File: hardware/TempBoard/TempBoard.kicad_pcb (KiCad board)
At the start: 2 copper layers, 27.1 x 27.1 mm, 17 parts, among them J1 Conn_01x04, J2 Conn_01x03, U1 BME280

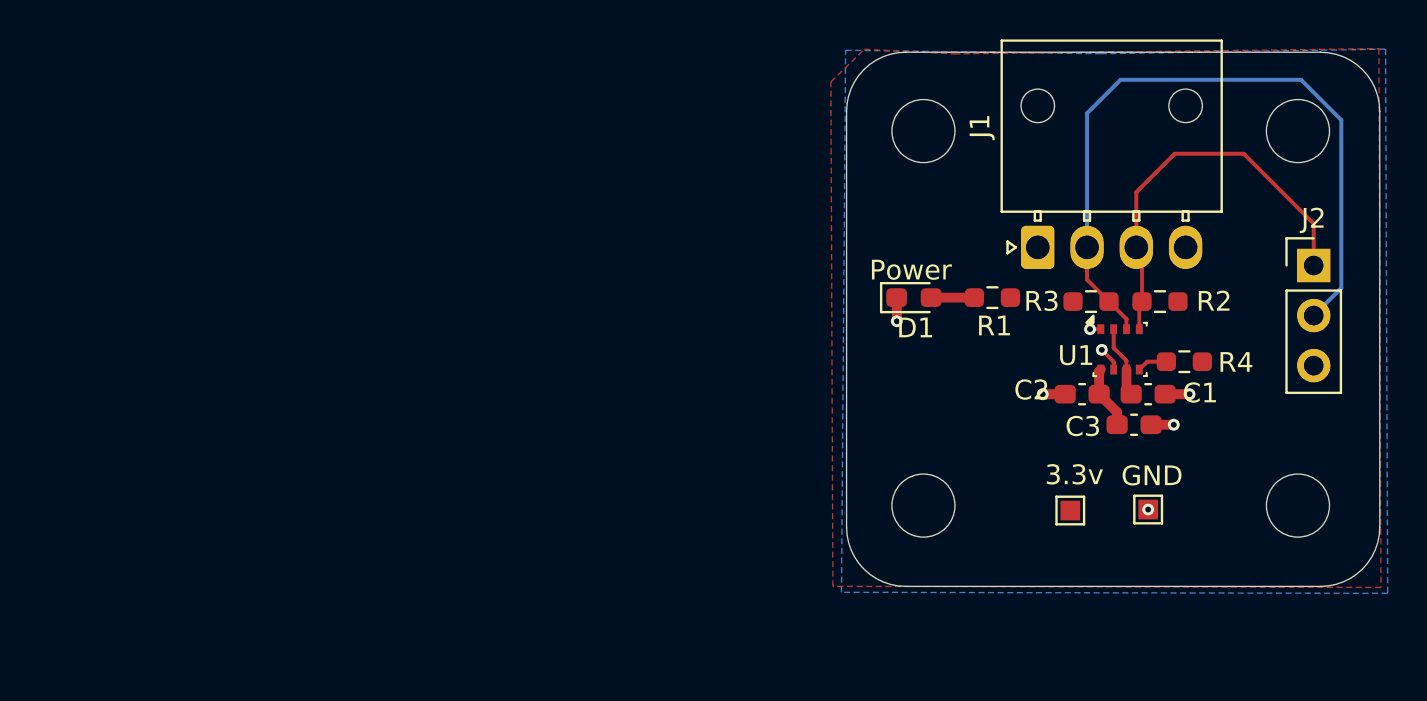
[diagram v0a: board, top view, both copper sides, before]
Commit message: pitot board ordered, routing+size finished for temperature board so pull??
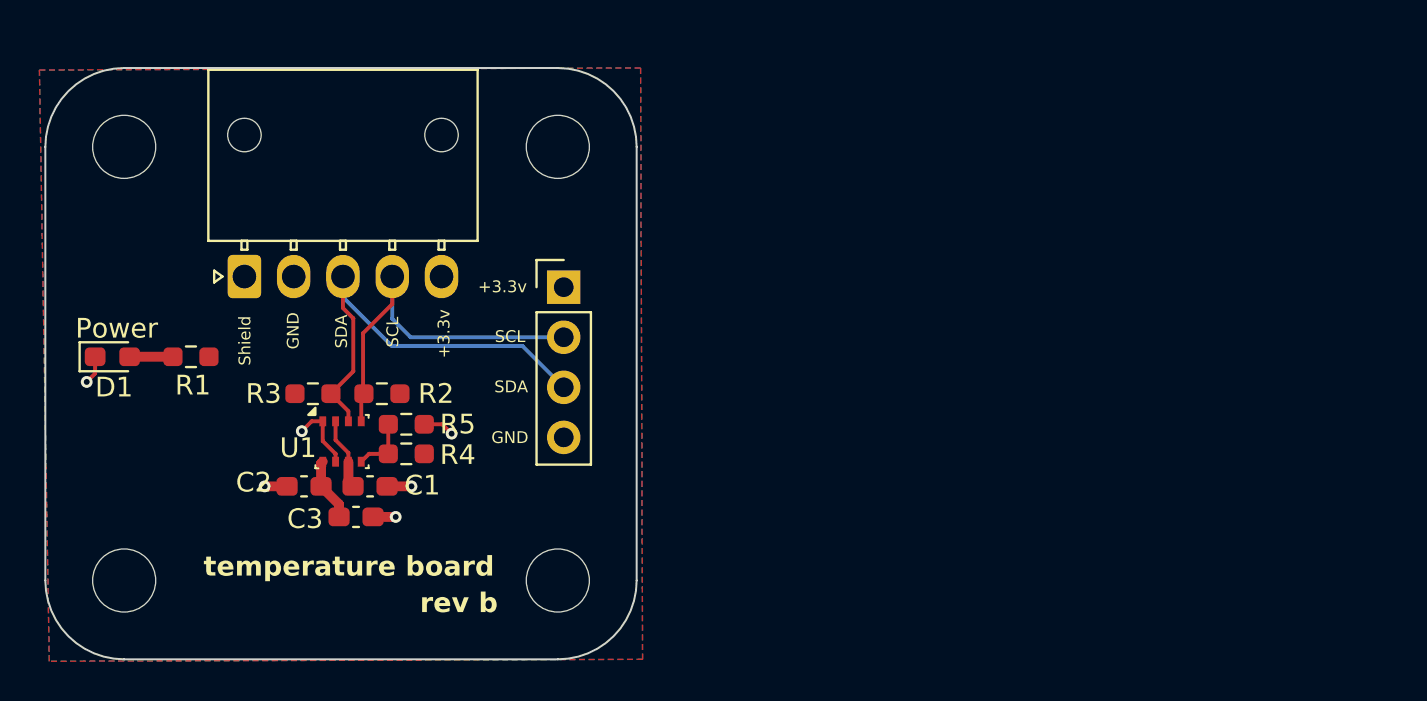
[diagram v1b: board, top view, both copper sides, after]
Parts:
- removed 3.3v, GND: TestPoint, TestPoint:TestPoint_Pad_1.0x1.0mm
- removed J1: Conn_01x04, Connector_Molex:Molex_Nano-Fit_105313-xx04_1x04_P2.50mm_Horizontal
- added J3: Conn_01x05, Connector_Molex:Molex_Nano-Fit_105313-xx05_1x05_P2.50mm_Horizontal, F.Cu at (125.8, 64.5)
- added R5: 0, Resistor_SMD:R_0603_1608Metric_Pad0.98x0.95mm_HandSolder, F.Cu at (134.0, 72.0)
- J2: value Conn_01x03 -> Conn_01x04; footprint Connector_PinHeader_2.54mm:PinHeader_1x03_P2.54mm_Vertical -> Connector_PinHeader_2.54mm:PinHeader_1x04_P2.54mm_Vertical
- R2, R3: value 4.6k -> 4.7k
- moved H4 59.7 mm to (119.7, 79.9)
- moved H2 43.9 mm to (141.7, 79.9)
- moved D1 40.8 mm to (119.1, 68.5)
- moved R1 40.8 mm to (123.1, 68.5)
- moved H1 40.6 mm to (119.7, 57.9)
- moved C2 39.8 mm to (128.8, 75.1)
- moved R4 39.8 mm to (134.0, 73.5)
- moved C1 39.8 mm to (132.2, 75.1)
- moved C3 39.8 mm to (131.5, 76.7)
- moved R2 39.8 mm to (132.8, 70.4)
- moved R3 39.8 mm to (129.3, 70.4)
- moved U1 39.8 mm to (130.8, 72.8)
- moved J2 38.1 mm to (142.0, 65.0)
- moved H3 26.0 mm to (141.7, 57.9)
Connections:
- J2 pad 1: /SCL -> +3.3V
- J2 pad 2: /SDA -> /SCL
- J2 pad 3: GND -> /SDA
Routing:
- net /SDA: track 36.7 -> 23.9 mm
- net GND: track 6.53 -> 10.2 mm, vias 7 -> 6
- net Net-(U1-SDO): track 1.54 -> 3.04 mm
- net /SCL: track 20.5 -> 19.7 mm
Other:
- board size 27.1 x 27.1 mm -> 30 x 30 mm
- board text added: "+3.3v"
- board text added: "GND"
- board text added: "Karthik Kurapati Febuary 2026"
- board text added: "SCL"
- board text added: "SDA"
- board text added: "Shield"
- board text added: "rev b"
- board text added: "temperature board"
